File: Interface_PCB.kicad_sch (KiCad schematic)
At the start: 25 parts, among them IC1 STM32L412RBT6P, J1 USB_B, J2 AVR-JTAG-10, J3 Conn_01x04, J4 Conn_01x04, J5 Conn_01x04, J6 Conn_01x04, U1 AMS1117, Y1 Crystal, Y2 Crystal

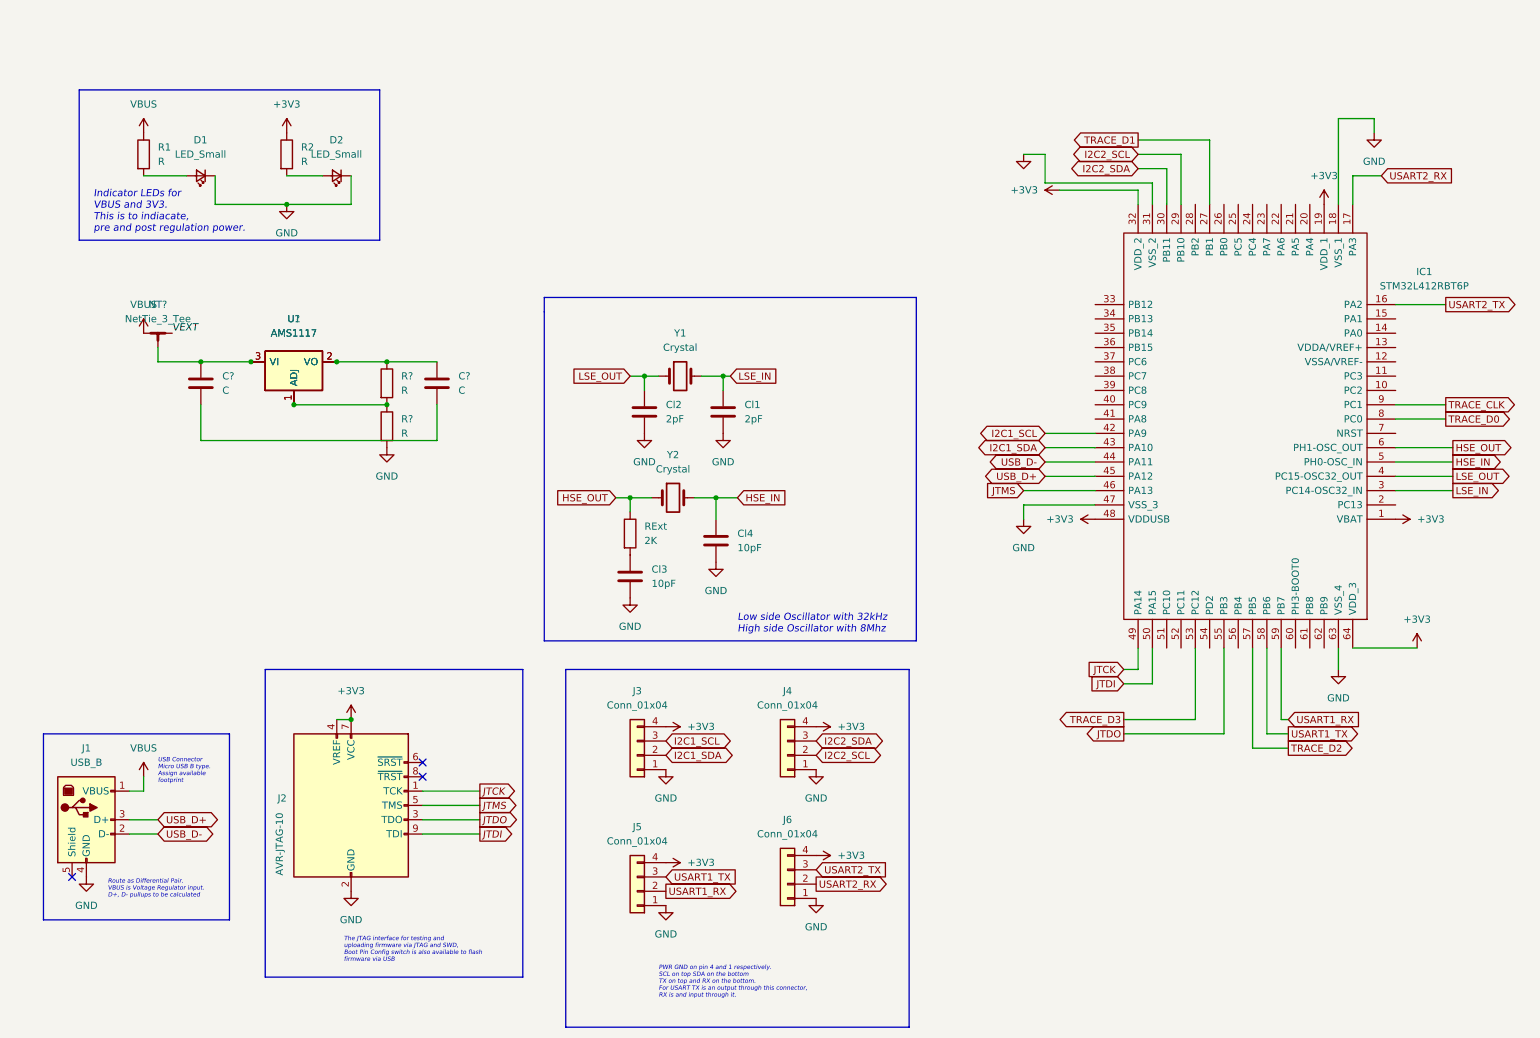
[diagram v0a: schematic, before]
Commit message: Final Schematic done, footprint assignment TBD
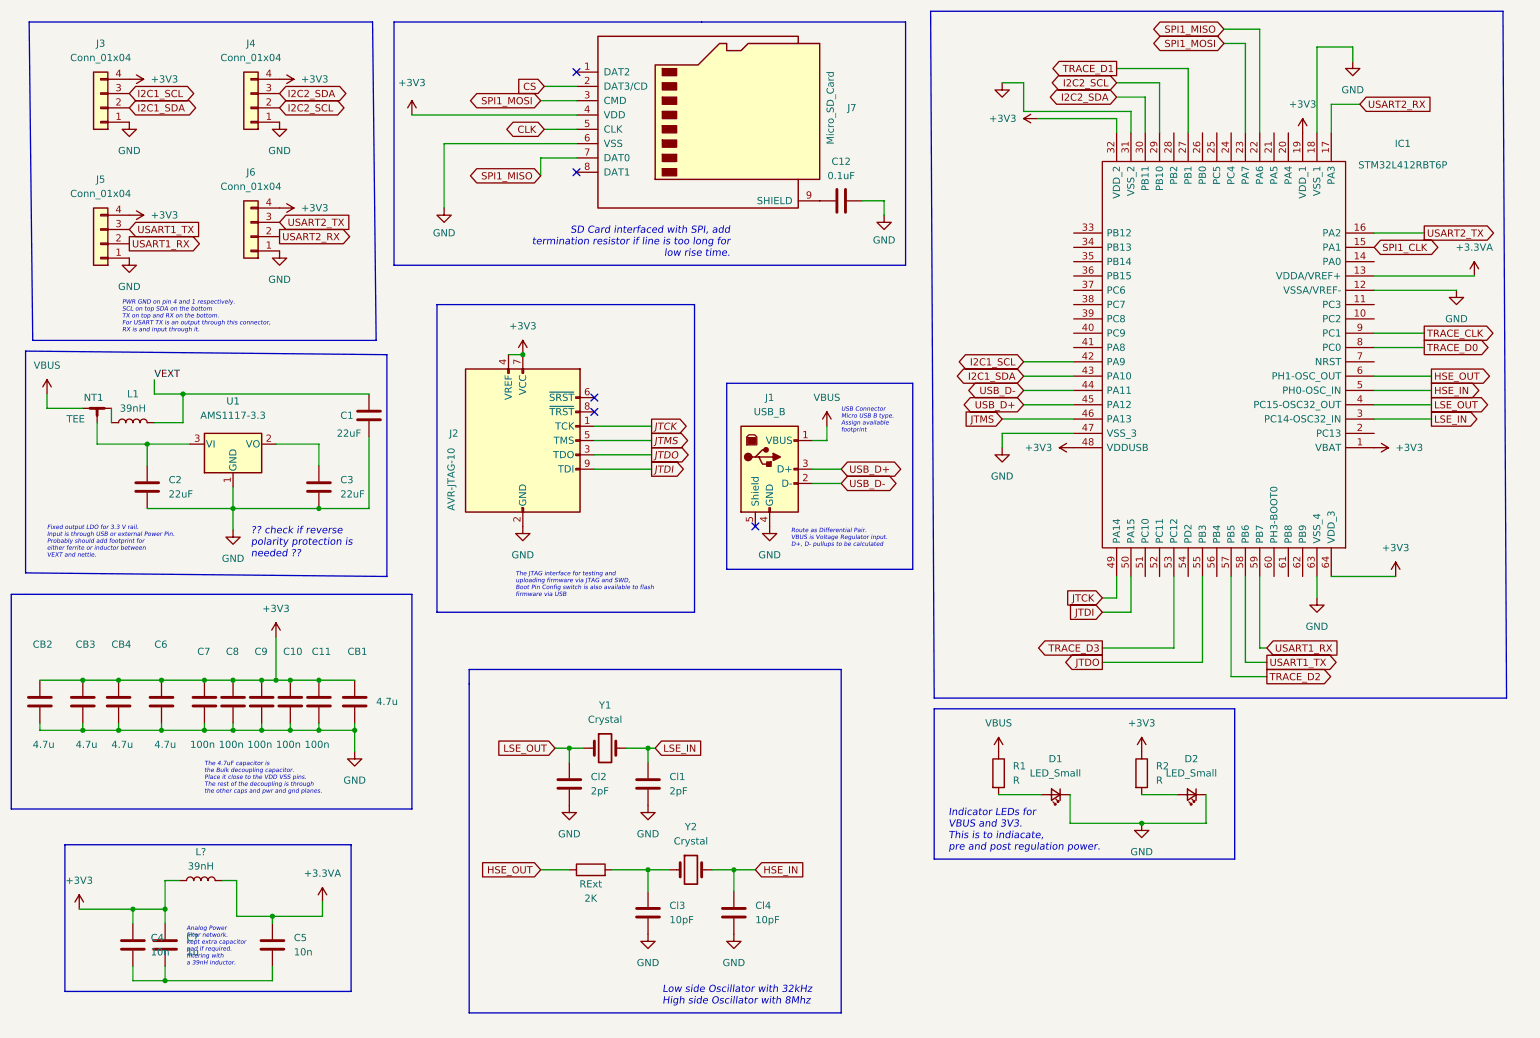
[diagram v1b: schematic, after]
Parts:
- removed C? (x2): C, symbol Device:C
- removed NT?: NetTie_3_Tee, symbol Device:NetTie_3_Tee
- removed R? (x2): R, symbol Device:R
- removed U1, U?: AMS1117, Package_TO_SOT_SMD:SOT-223-3_TabPin2, symbol Regulator_Linear:AMS1117
- added C1, C2, C3: 22uF, symbol Device:C
- added C10, C11, C7, C8, C9: 100n, symbol Device:C
- added C12: 0.1uF, symbol Device:C
- added C4, C5: 10n, symbol Device:C
- added C6, CB1, CB2, CB3, CB4: 4.7u, symbol Device:C
- added C?: 1u, symbol Device:C
- added J7: Micro_SD_Card, Connector_Card:microSD_HC_Wuerth_693072010801, symbol Connector:Micro_SD_Card
- added L1, L?: 39nH, symbol Device:L
- added NT1: TEE, symbol Device:NetTie_3_Tee
- added U1: AMS1117-3.3, Package_TO_SOT_SMD:SOT-223-3_TabPin2, symbol Regulator_Linear:AMS1117-3.3
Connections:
- net +3V3: now also C10.1, C11.1, C4.1, C6.1, C7.1, C8.1, C9.1, C?.1, CB1.1, CB2.1, CB3.1, CB4.1, J7.4 (VDD), L?.1
- net GND: now also IC1.12 (VSSA/VREF-), C1.2, C10.2, C11.2, C12.2, C2.2, C3.2, C6.2, C7.2, C8.2, C9.2, CB1.2, CB2.2, CB3.2, CB4.2, J7.6 (VSS), U1.1 (GND)
- net HSE_OUT: no longer Y2.1
- net VBUS: now also NT1.1
- net VEXT: now also C1.1, L1.2
- net at Cl3.1, RExt.2: now also Y2.1
- net +3.3VA: now reaches IC1.13 (VDDA/VREF+)
- net +3.3VA: now also C5.1, L?.2
- net SPI1_CLK: now reaches IC1.15 (PA1)
- net SPI1_MISO: now reaches IC1.22 (PA6)
- net SPI1_MISO: now also J7.7 (DAT0)
- net SPI1_MOSI: now reaches IC1.23 (PA7)
- net SPI1_MOSI: now also J7.3 (CMD)
- new net: C3.1, U1.2 (VO)
- new net: C12.1, J7.9 (SHIELD)
- new net: C2.1, NT1.3, U1.3 (VI)
- new net: C4.2, C5.2, C?.2
- new net: L1.1, NT1.2
- new net CLK: J7.5 (CLK)
- new net CS: J7.2 (DAT3/CD)
- no-connect marks 3 -> 5
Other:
- note added: "?? check if reverse polarity protection is needed ??"
- note added: "Analog Power filter network. kept extra capacitor pad if required. filtering with a 39nH inductor."
- note added: "Fixed output LDO for 3.3 V rail. Input is through USB or external Power Pin. Probably should add footprint for either ferrite or inductor between VEXT and nettie."
- note added: "SD Card interfaced with SPI, add termination resistor if line is too long for low rise time."
- note added: "The 4.7uF capacitor is the Bulk decoupling capacitor. Place it close to the VDD VSS pins. The rest of the decoupling is through the other caps and pwr and gnd planes."
- moved on the sheet: Cl1, Cl2, Cl3, Cl4, D1, D2, IC1, J1, J2, J3, J4, J5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
